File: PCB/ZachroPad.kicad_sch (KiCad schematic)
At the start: 7 parts, among them SW1 SW_Push, SW2 SW_Push, SW3 SW_Push, SW4 SW_Push, U1 XIAO-RP2040-DIP

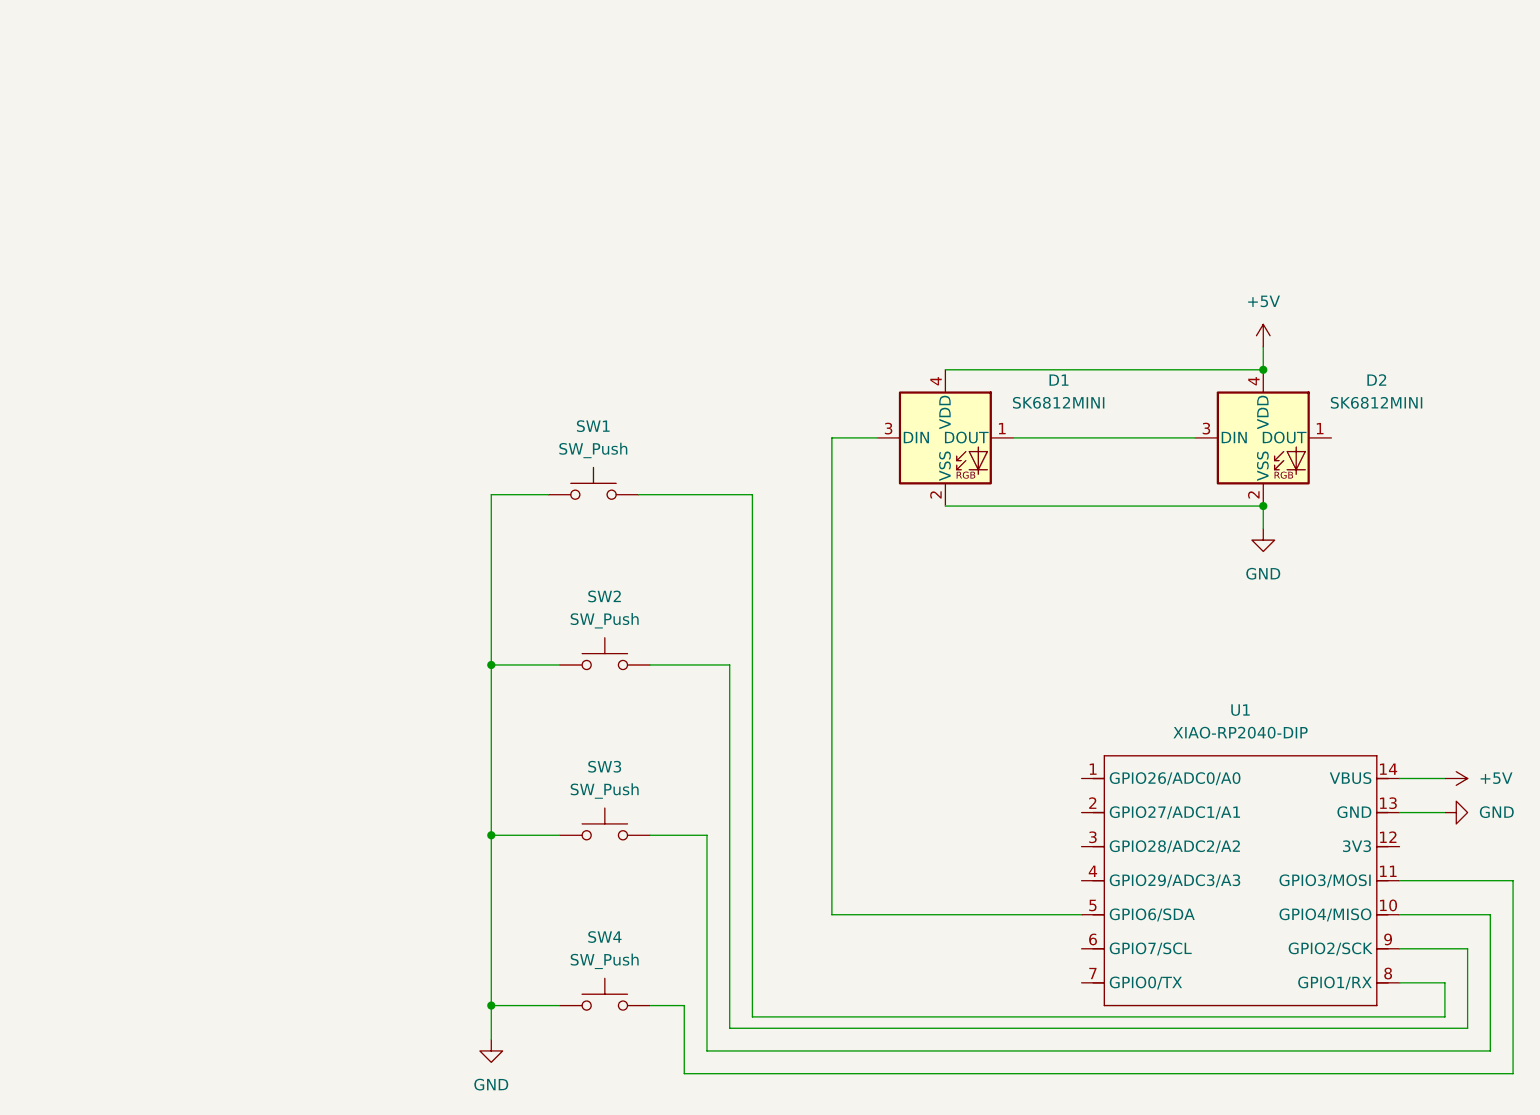
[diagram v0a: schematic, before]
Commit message: updates!
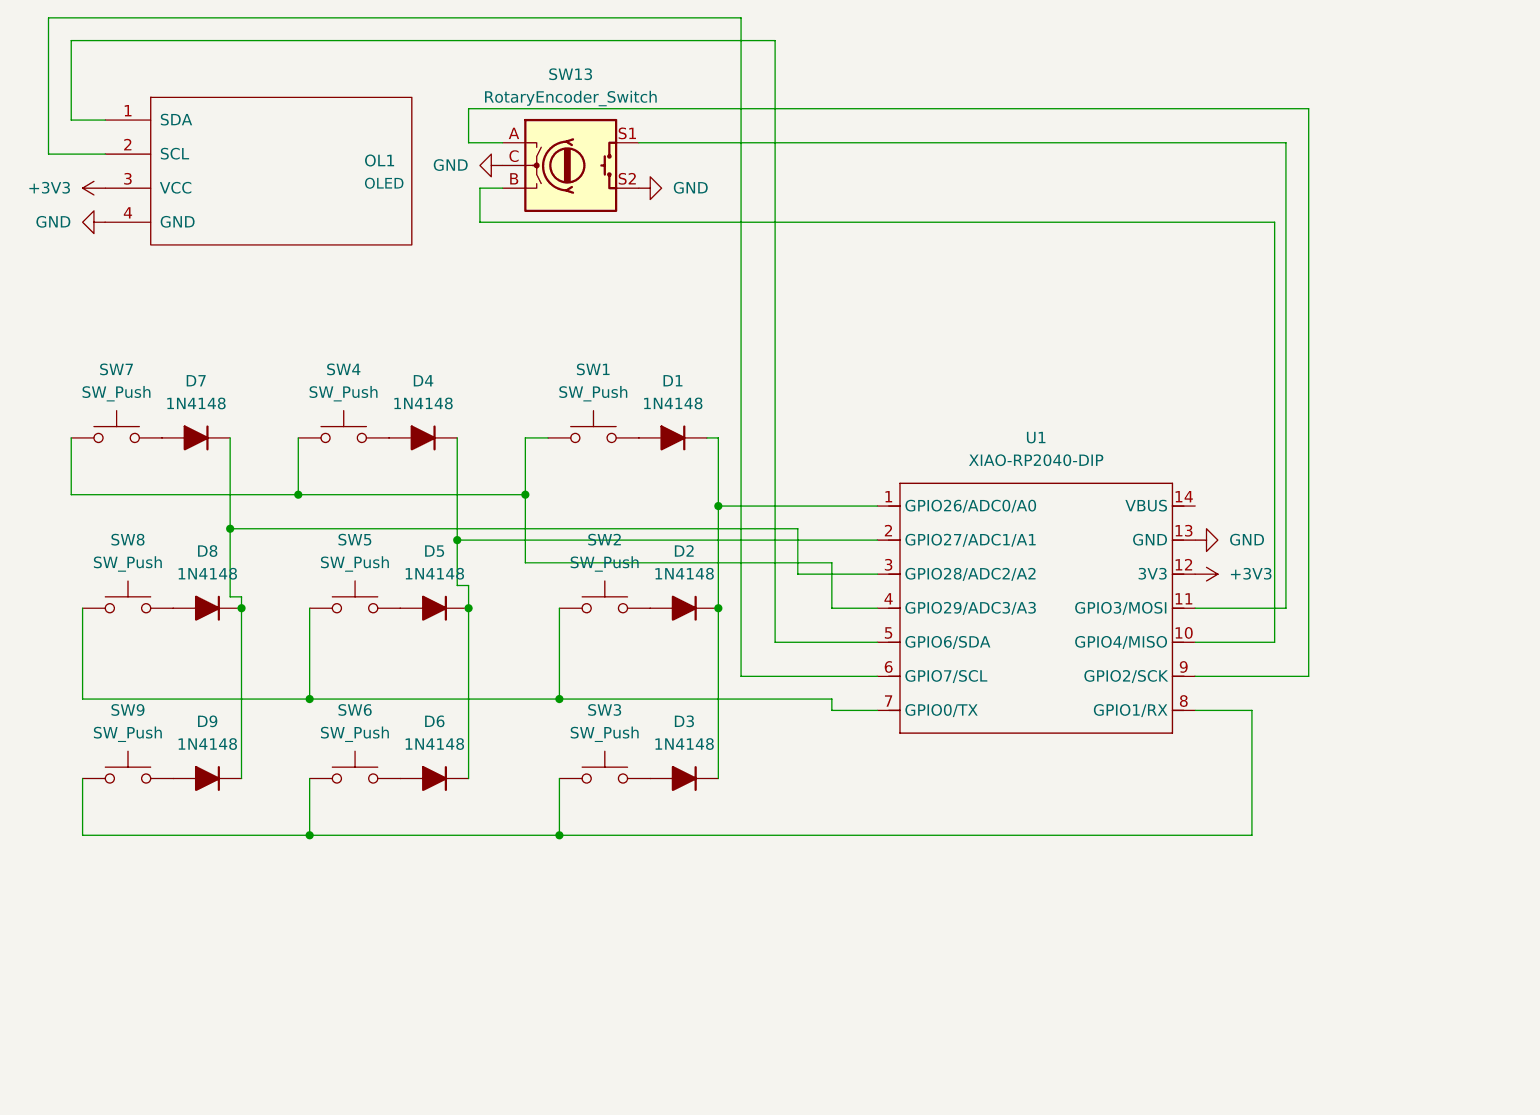
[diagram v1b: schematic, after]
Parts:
- removed D1, D2: SK6812MINI, PCM_LED_SMD_AKL:LED_SK6812MINI_PLCC4_3.5x3.5mm_P1.75mm, symbol LED:SK6812MINI
- added D1, D2, D3, D4, D5, D6, D7, D8, D9: 1N4148, PCM_Diode_THT_AKL:D_DO-35_SOD27_P7.62mm_Horizontal, symbol PCM_Diode_AKL:1N4148
- added OL1: OLED, OLED:SSD1306-0.91-OLED-4pin-128x32, symbol OLED:OLED
- added SW13: RotaryEncoder_Switch, Rotary Encoder:RotaryEncoder_Alps_EC11E-Switch_Vertical_H20mm, symbol Device:RotaryEncoder_Switch
- added SW5, SW6, SW7, SW8, SW9: SW_Push, PCM_Switch_Keyboard_Cherry_MX:SW_Cherry_MX_PCB_1.00u, symbol Switch:SW_Push
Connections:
- net GND: now also OL1.4 (GND), SW13.C, SW13.S2; no longer SW1.1, SW2.1, SW3.1, SW4.1
- net at SW2.2: now also D2.2 (A); no longer U1.9 (GPIO2/SCK)
- net at U1.10 (GPIO4/MISO): now also SW13.B; no longer SW3.2
- net at SW4.2: now also D4.2 (A); no longer U1.11 (GPIO3/MOSI)
- net at U1.1 (GPIO26/ADC0/A0): now also D1.1 (K), D2.1 (K), D3.1 (K)
- net +3V3: now reaches U1.12 (3V3)
- net +3V3: now also OL1.3 (VCC)
- net at U1.2 (GPIO27/ADC1/A1): now also D4.1 (K), D5.1 (K), D6.1 (K)
- net at U1.3 (GPIO28/ADC2/A2): now also D7.1 (K), D8.1 (K), D9.1 (K)
- net at U1.4 (GPIO29/ADC3/A3): now also SW1.1, SW4.1, SW7.1
- net at U1.5 (GPIO6/SDA): now also OL1.1 (SDA)
- net at U1.6 (GPIO7/SCL): now also OL1.2 (SCL)
- net at U1.7 (GPIO0/TX): now also SW2.1, SW5.1, SW8.1
- net at SW1.2: now also D1.2 (A); no longer U1.8 (GPIO1/RX)
- net +5V: no longer names the net of U1.14 (VBUS)
- new net: D8.2 (A), SW8.2
- new net: SW13.A, U1.9 (GPIO2/SCK)
- new net: SW13.S1, U1.11 (GPIO3/MOSI)
- new net: SW3.1, SW6.1, SW9.1, U1.8 (GPIO1/RX)
- new net: D6.2 (A), SW6.2
- new net: D3.2 (A), SW3.2
- new net: D5.2 (A), SW5.2
- new net: D7.2 (A), SW7.2
- new net: D9.2 (A), SW9.2
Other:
- moved on the sheet: SW1, SW2, SW3, U1
